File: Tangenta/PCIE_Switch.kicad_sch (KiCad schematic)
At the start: 99 parts, among them U15 PI7C9X2G404SLBFDEX, U17 M24C04-RMN6TP

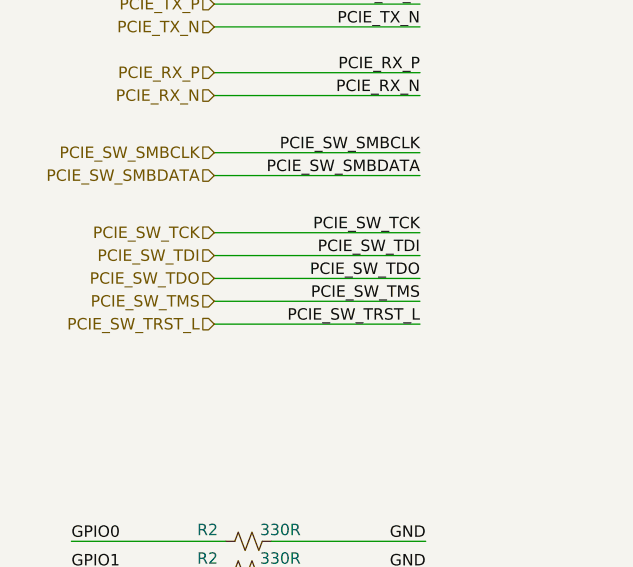
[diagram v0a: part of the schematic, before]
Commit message: Schematic improvements.
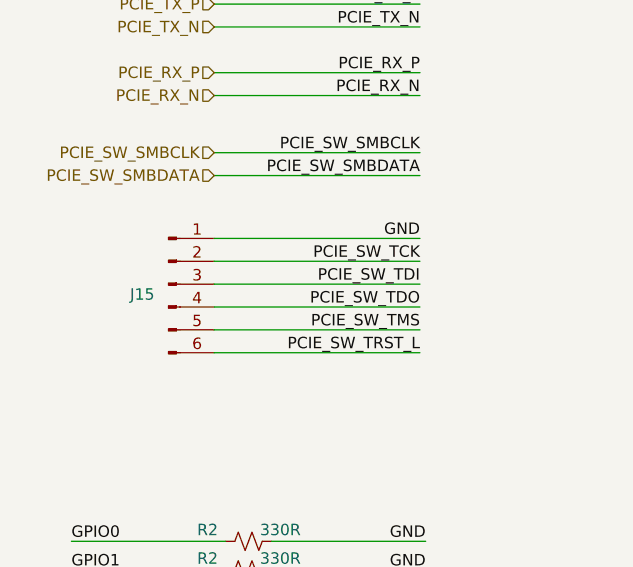
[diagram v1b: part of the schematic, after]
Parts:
- added J15: Conn_01x06_Pin, Connector_PinHeader_1.00mm:PinHeader_1x06_P1.00mm_Vertical, symbol Connector:Conn_01x06_Pin
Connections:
- net GNDREF: now also J15.1 (Pin_1)
- net PCIE_SW_TCK: now also J15.2 (Pin_2)
- net PCIE_SW_TDI: now also J15.3 (Pin_3)
- net PCIE_SW_TDO: now also J15.4 (Pin_4)
- net PCIE_SW_TMS: now also J15.5 (Pin_5)
- net PCIE_SW_TRST_L: now also J15.6 (Pin_6)
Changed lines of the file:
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@@
     (stroke (width 0) (type default))
   )
+  (wire (pts (xy 34.29 97.155) (xy 57.15 97.155))
+    (stroke (width 0) (type default))
+  )
   (wire (pts (xy 35.56 135.255) (xy 18.415 135.255))
     (stroke (width 0) (type default))
@@
     (stroke (width 0) (type default))
   )
+  (wire (pts (xy 34.29 102.235) (xy 57.15 102.235))
+    (stroke (width 0) (type default))
+  )
   (wire (pts (xy 382.905 223.52) (xy 400.05 223.52))
     (stroke (width 0) (type default))
@@
     (stroke (width 0) (type default))
   )
-  (wire (pts (xy 233.68 161.29) (xy 248.92 161.29))
+  (wire (pts (xy 34.29 99.695) (xy 57.15 99.695))
     (stroke (width 0) (type default))
   )
-  (wire (pts (xy 180.34 218.44) (xy 165.1 218.44))
+  (wire (pts (xy 233.68 161.29) (xy 248.92 161.29))
     (stroke (width 0) (type default))
   )
-  (wire (pts (xy 57.15 99.06) (xy 34.29 99.06))
+  (wire (pts (xy 180.34 218.44) (xy 165.1 218.44))
     (stroke (width 0) (type default))
   )
@@
     (stroke (width 0) (type default))
   )
-  (wire (pts (xy 57.15 91.44) (xy 34.29 91.44))
-    (stroke (width 0) (type default))
-  )
   (wire (pts (xy 363.22 93.98) (xy 363.22 96.52))
     (stroke (width 0) (type default))
@@
     (stroke (width 0) (type default))
   )
+  (wire (pts (xy 34.29 92.075) (xy 57.15 92.075))
+    (stroke (width 0) (type default))
+  )
   (wire (pts (xy 35.56 264.795) (xy 18.415 264.795))
     (stroke (width 0) (type default))
@@
     (stroke (width 0) (type default))
   )
-  (wire (pts (xy 57.15 93.98) (xy 34.29 93.98))
-    (stroke (width 0) (type default))
-  )
   (wire (pts (xy 379.73 115.57) (xy 379.73 118.11))
     (stroke (width 0) (type default))
@@
     (stroke (width 0) (type default))
   )
+  (wire (pts (xy 34.29 104.775) (xy 57.15 104.775))
+    (stroke (width 0) (type default))
+  )
   (wire (pts (xy 213.36 267.97) (xy 232.41 267.97))
     (stroke (width 0) (type default))
@@
     (stroke (width 0) (type default))
   )
-  (wire (pts (xy 57.15 101.6) (xy 34.29 101.6))
-    (stroke (width 0) (type default))
-  )
   (wire (pts (xy 18.415 177.165) (xy 35.56 177.165))
     (stroke (width 0) (type default))
@@
     (stroke (width 0) (type default))
   )
-  (wire (pts (xy 57.15 96.52) (xy 34.29 96.52))
-    (stroke (width 0) (type default))
-  )
   (wire (pts (xy 180.34 139.7) (xy 165.1 139.7))
     (stroke (width 0) (type default))
@@
     (stroke (width 0) (type default))
   )
+  (wire (pts (xy 34.29 94.615) (xy 57.15 94.615))
+    (stroke (width 0) (type default))
+  )
   (wire (pts (xy 389.89 22.86) (xy 389.89 25.4))
     (stroke (width 0) (type default))
@@
     (effects (font (size 1.27 1.27)) (justify right bottom))
   )
-  (label "PCIE_SW_TRST_L" (at 57.15 101.6 180) (fields_autoplaced)
+  (label "PCIE_SW_TRST_L" (at 57.15 104.775 180) (fields_autoplaced)
     (effects (font (size 1.27 1.27)) (justify right bottom))
   )
@@
     (effects (font (size 1.27 1.27)) (justify left bottom))
   )
+  (label "GND" (at 57.15 92.075 180) (fields_autoplaced)
+    (effects (font (size 1.27 1.27)) (justify right bottom))
+  )
   (label "1V0" (at 318.77 93.98 0) (fields_autoplaced)
     (effects (font (size 1.27 1.27)) (justify left bottom))
@@
     (effects (font (size 1.27 1.27)) (justify left bottom))
   )
-  (label "PCIE_SW_TCK" (at 57.15 91.44 180) (fields_autoplaced)
+  (label "PCIE_SW_TCK" (at 57.15 94.615 180) (fields_autoplaced)
     (effects (font (size 1.27 1.27)) (justify right bottom))
   )
@@
     (effects (font (size 1.27 1.27)) (justify left bottom))
   )
-  (label "PCIE_SW_TDO" (at 57.15 96.52 180) (fields_autoplaced)
+  (label "PCIE_SW_TDO" (at 57.15 99.695 180) (fields_autoplaced)
     (effects (font (size 1.27 1.27)) (justify right bottom))
   )
@@
     (effects (font (size 1.27 1.27)) (justify left bottom))
   )
-  (label "PCIE_SW_TMS" (at 57.15 99.06 180) (fields_autoplaced)
+  (label "PCIE_SW_TMS" (at 57.15 102.235 180) (fields_autoplaced)
     (effects (font (size 1.27 1.27)) (justify right bottom))
   )
@@
     (effects (font (size 1.27 1.27)) (justify left bottom))
   )
-  (label "PCIE_SW_TDI" (at 57.15 93.98 180) (fields_autoplaced)
+  (label "PCIE_SW_TDI" (at 57.15 97.155 180) (fields_autoplaced)
     (effects (font (size 1.27 1.27)) (justify right bottom))
   )
@@
     (effects (font (size 1.27 1.27)) (justify left bottom))
   )
-  (hierarchical_label "PCIE_SW_TDO" (shape input) (at 34.29 96.52 180) (fields_autoplaced)
-    (effects (font (size 1.27 1.27)) (justify right))
-  )
   (hierarchical_label "PCIE1_CLK_N" (shape output) (at 386.715 139.7 0) (fields_autoplaced)
     (effects (font (size 1.27 1.27)) (justify left))
@@
     (effects (font (size 1.27 1.27)) (justify left))
   )
-  (hierarchical_label "PCIE_SW_TCK" (shape input) (at 34.29 91.44 180) (fields_autoplaced)
-    (effects (font (size 1.27 1.27)) (justify right))
-  )
   (hierarchical_label "PCIE3_PRSNT" (shape output) (at 386.715 190.5 0) (fields_autoplaced)
     (effects (font (size 1.27 1.27)) (justify left))
@@
     (effects (font (size 1.27 1.27)) (justify left))
   )
-  (hierarchical_label "PCIE_SW_TMS" (shape input) (at 34.29 99.06 180) (fields_autoplaced)
-    (effects (font (size 1.27 1.27)) (justify right))
-  )
   (hierarchical_label "PCIE2_CLK_N" (shape output) (at 386.715 168.91 0) (fields_autoplaced)
     (effects (font (size 1.27 1.27)) (justify left))
@@
     (effects (font (size 1.27 1.27)) (justify left))
   )
-  (hierarchical_label "PCIE_SW_TDI" (shape input) (at 34.29 93.98 180) (fields_autoplaced)
-    (effects (font (size 1.27 1.27)) (justify right))
-  )
-  (hierarchical_label "PCIE_SW_TRST_L" (shape input) (at 34.29 101.6 180) (fields_autoplaced)
-    (effects (font (size 1.27 1.27)) (justify right))
-  )
   (hierarchical_label "PCIE_RX_P" (shape input) (at 34.29 73.66 180) (fields_autoplaced)
     (effects (font (size 1.27 1.27)) (justify right))
@@
         )
       )
+    )
+  )
+  (symbol (lib_id "Connector:Conn_01x06_Pin") (at 29.21 97.155 0) (unit 1)
+    (in_bom yes) (on_board yes) (dnp no)
+    (property "Reference" "J15" (at 26.289 98.298 0)
+      (effects (font (size 1.27 1.27)))
+    )
+    (property "Value" "Conn_01x06_Pin" (at 29.845 89.535 0)
+      (effects (font (size 1.27 1.27)) hide)
+    )
+    (property "Footprint" "Connector_PinHeader_1.00mm:PinHeader_1x06_P1.00mm_Vertical" (at 29.21 97.155 0)
+      (effects (font (size 1.27 1.27)) hide)
+    )
+    (property "Datasheet" "~" (at 29.21 97.155 0)
+      (effects (font (size 1.27 1.27)) hide)
+    )
+    (pin "1")
+    (pin "2")
+    (pin "3")
+    (pin "4")
+    (pin "5")
+    (pin "6")
+    (instances
+      (project "Tangenta"
+        (path "/358d1bcf-7599-4352-8c4d-baa18a5f09e6/db297b0b-35f2-4e86-892c-83973f1ac2db"
+          (reference "J15") (unit 1)
+        )
+        (path "/358d1bcf-7599-4352-8c4d-baa18a5f09e6/9b1f6f94-444c-4c59-8de9-290bde336856/04648235-6c5e-4915-ab80-8fea22048f3c"
+          (reference "J15") (unit 1)
+        )
+      )
